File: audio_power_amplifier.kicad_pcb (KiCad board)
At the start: 2 copper layers, 190.7 x 90.9 mm, 95 parts, among them Q1 BC546, Q10 BC546, Q11 BC546, Q12 BC546, Q13 MJE15035, Q14 BC546, Q15 MJE15034, Q16 MJE15035, Q17 MJL4302, Q18 MJL4281, Q2 BC546, Q3 BC546, Q4 MJE15035, Q5 BC546, Q6 MJE15034, Q7 MJE15035, Q8 MJL4302, Q9 MJL4281

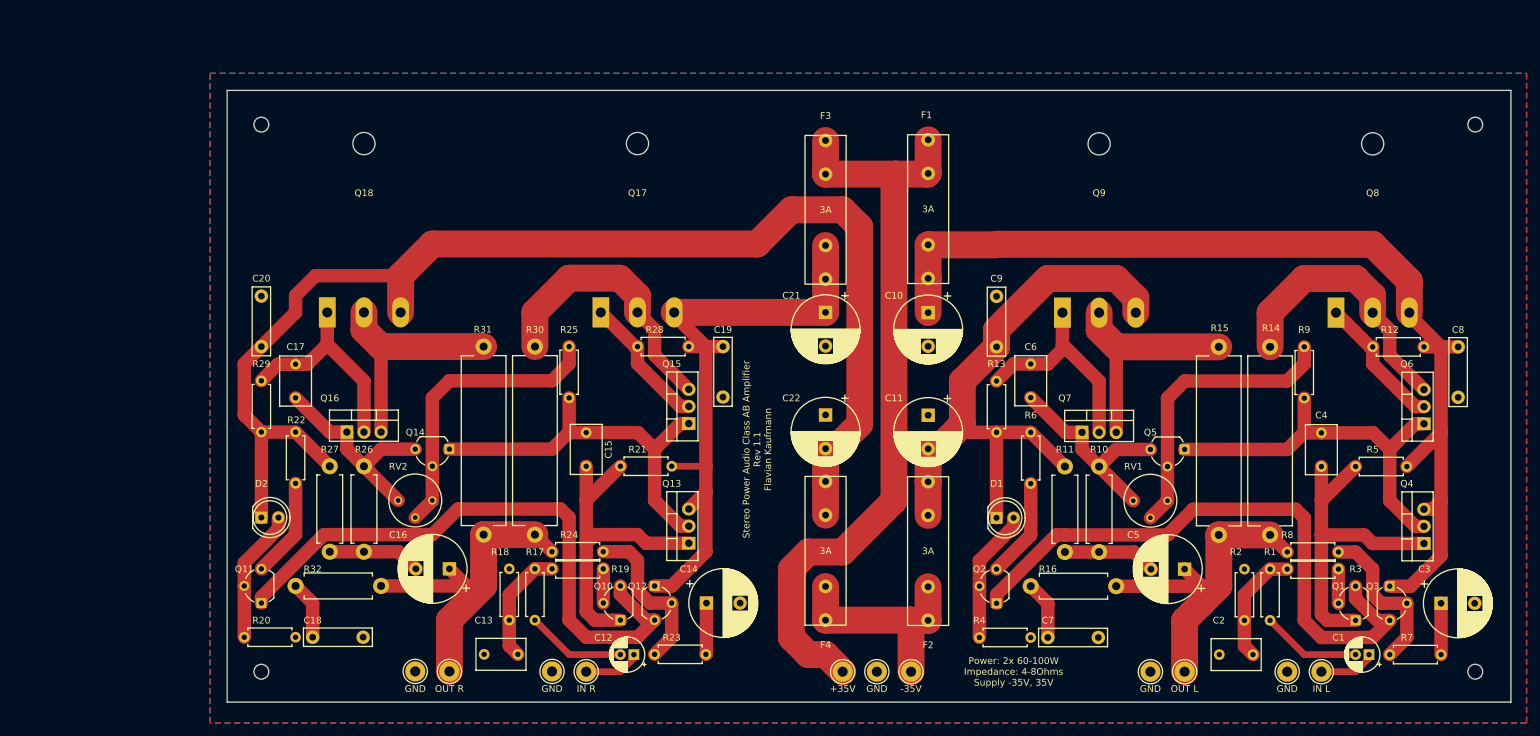
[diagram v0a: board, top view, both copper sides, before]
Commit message: cosmetics
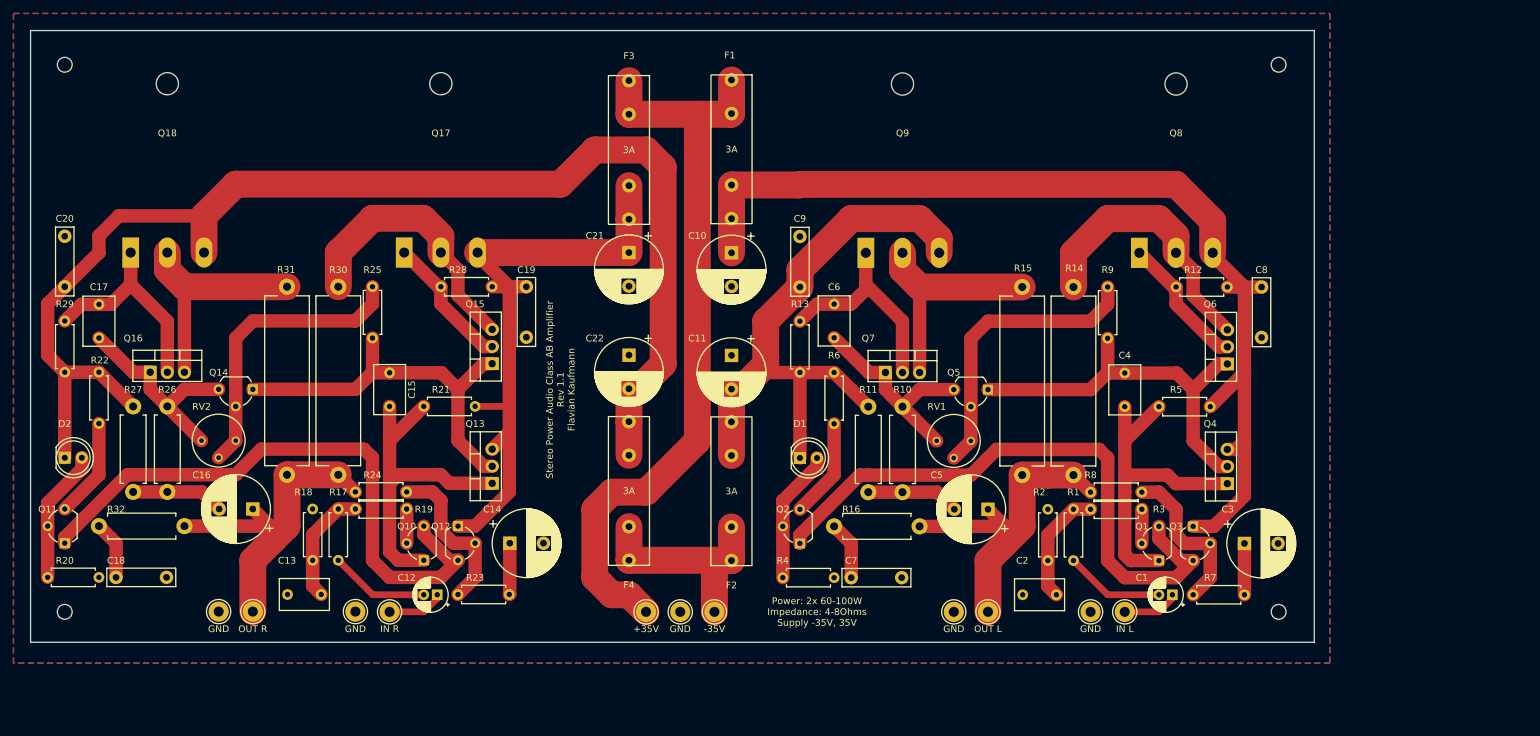
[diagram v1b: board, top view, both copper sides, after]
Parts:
- moved REF** 30.5 mm to (234.9, 57.1)
- moved REF** 30.5 mm to (234.9, 138.4)
- moved C1 30.5 mm to (219.2, 135.9)
- moved C13 30.5 mm to (92.7, 135.8)
- moved C7 30.5 mm to (171.4, 133.3)
- moved Q12 30.5 mm to (113.0, 125.7)
- moved Q4 30.5 mm to (227.3, 119.4)
- moved R1 30.5 mm to (204.5, 123.2)
- moved R23 30.5 mm to (113.0, 135.8)
- moved R3 30.5 mm to (207.0, 123.2)
- moved R4 30.5 mm to (168.9, 133.3)
- moved R7 30.5 mm to (222.2, 135.9)
- moved REF** 30.5 mm to (82.5, 138.4)
- moved REF** 30.5 mm to (77.5, 138.4)
- moved C10 30.5 mm to (153.7, 85.1)
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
